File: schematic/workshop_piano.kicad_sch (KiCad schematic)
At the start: 37 parts, among them J1 Jack-DC, J2 Conn_01x05_Pin, J3 AudioJack3, SW1 SW_SPST, SW2 SW_SPST, SW3 SW_SPST, SW4 SW_SPST, SW5 SW_SPST, SW6 SW_SPST, SW7 SW_SPST, SW8 SW_SPST, U1 PIC16F1459-IP

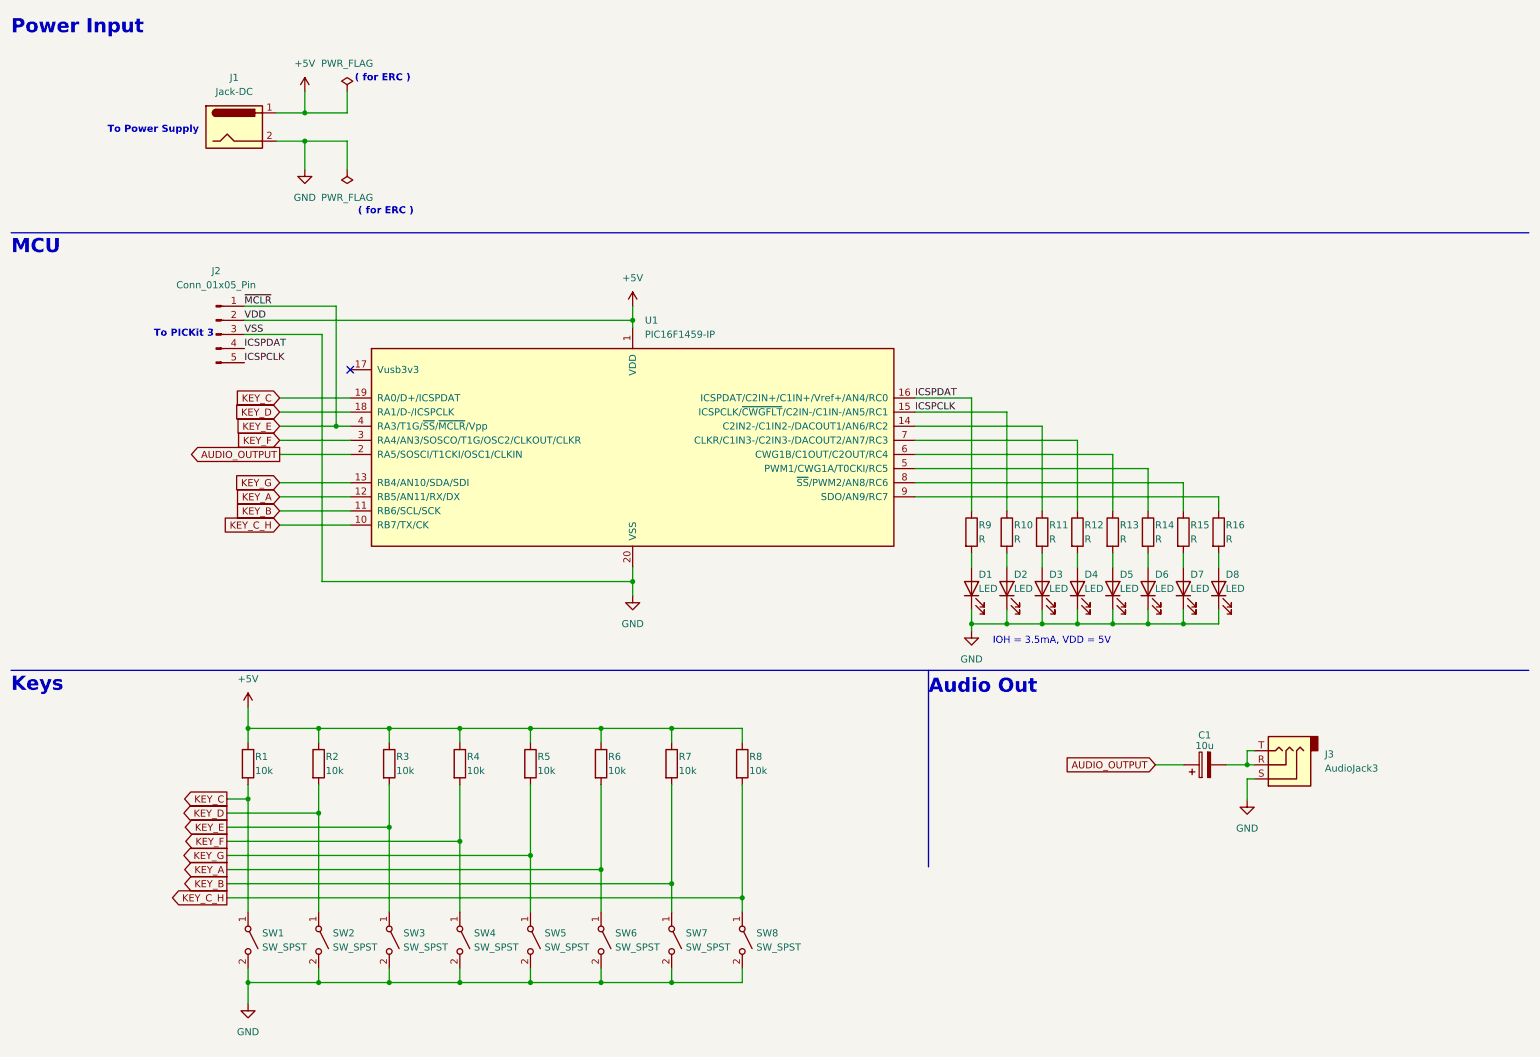
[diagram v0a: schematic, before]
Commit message: Update schematic
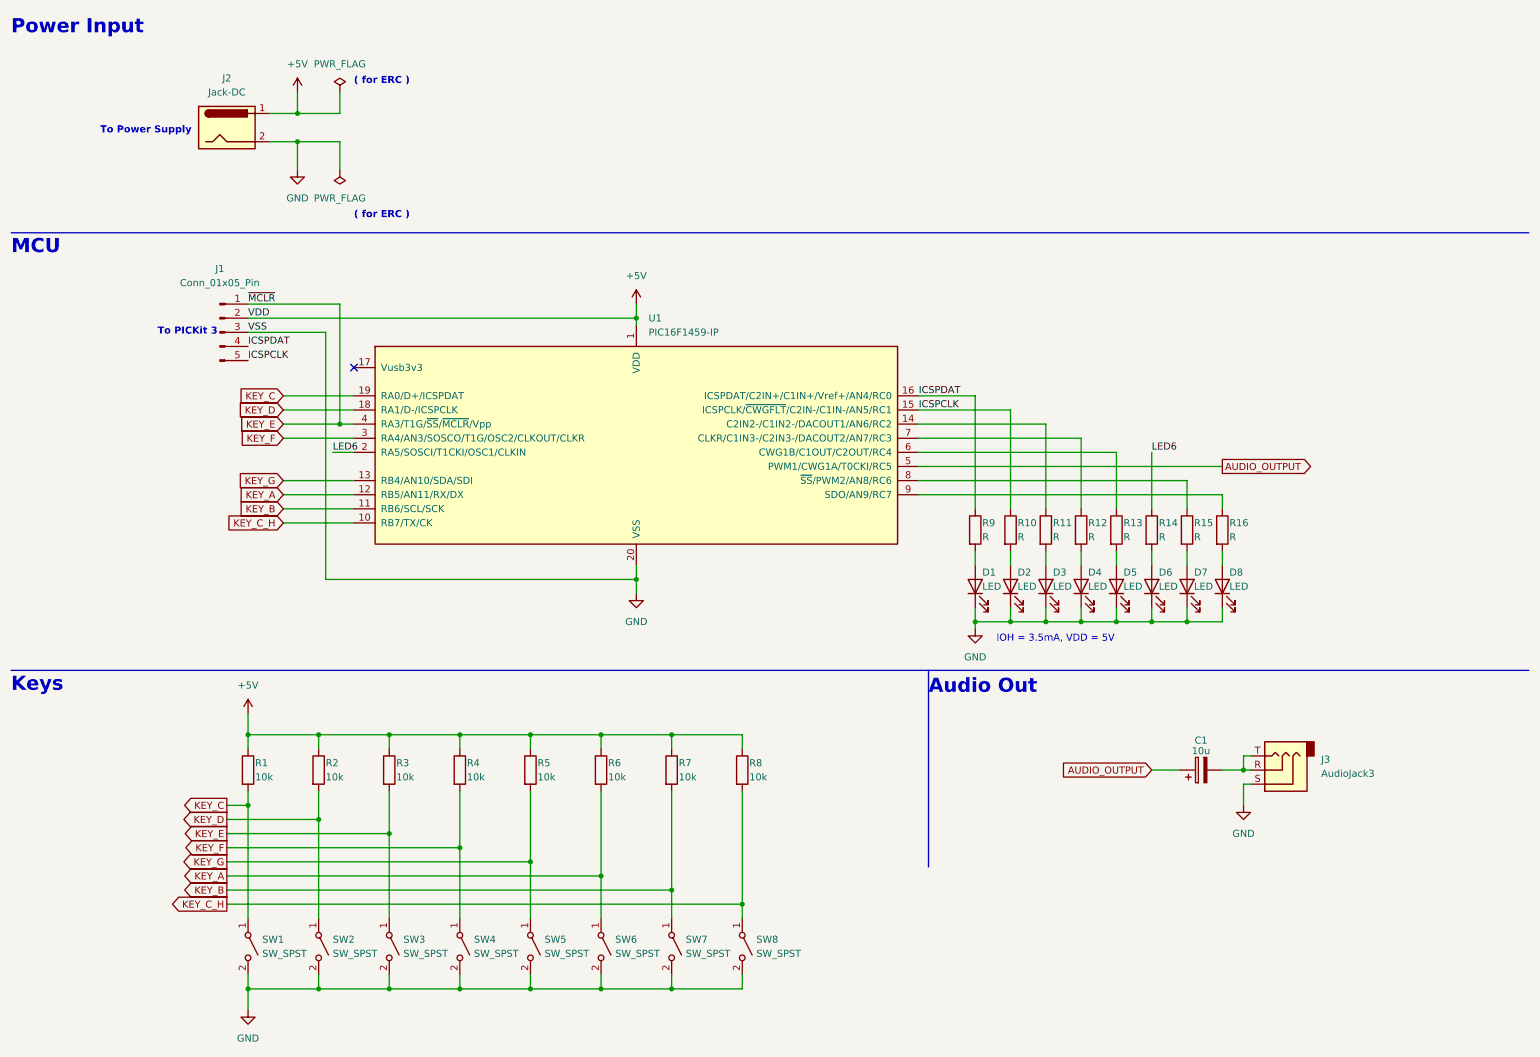
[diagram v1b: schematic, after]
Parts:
- renumbered J2 to J1, J1 to J2
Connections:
- net AUDIO_OUTPUT: now also U1.5 (PWM1/CWG1A/T0CKI/RC5); no longer U1.2 (RA5/SOSCI/T1CKI/OSC1/CLKIN)
- net LED6: now reaches R14.1
- net LED6: now also U1.2 (RA5/SOSCI/T1CKI/OSC1/CLKIN); no longer U1.5 (PWM1/CWG1A/T0CKI/RC5)
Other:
- moved on the sheet: C1, D1, D2, D3, D4, D5, D7, D8, J1, J2, J3, R1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
